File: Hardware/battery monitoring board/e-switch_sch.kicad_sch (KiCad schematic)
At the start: 8 parts, among them J5 Conn_01x02, K1 Relay_SPST-NO, Q2 PN2222A

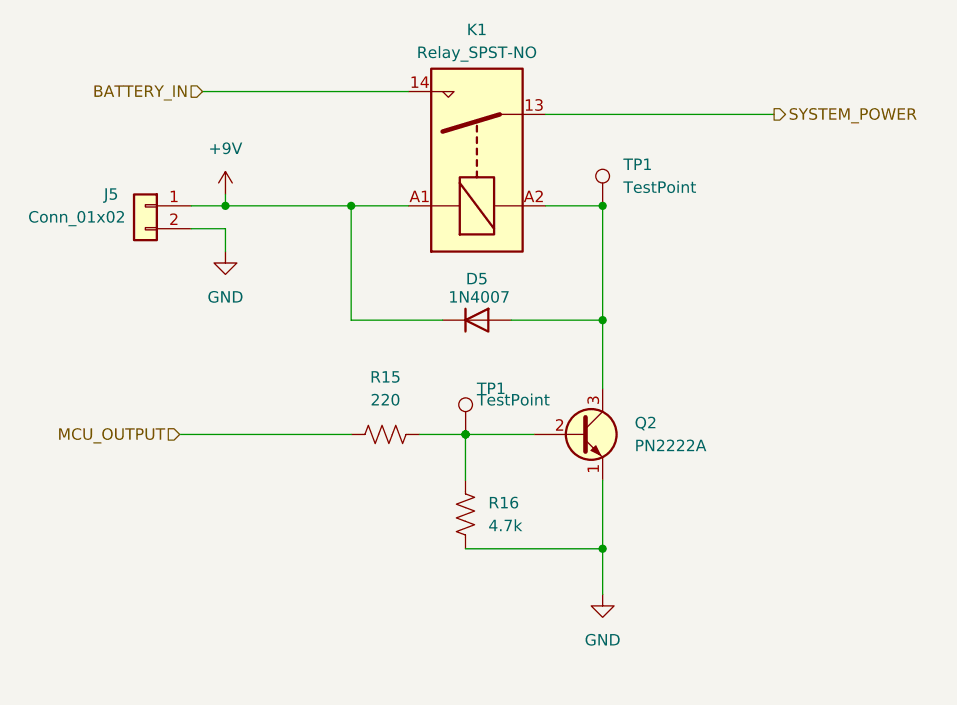
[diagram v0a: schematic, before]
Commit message: updated battery board pt.II
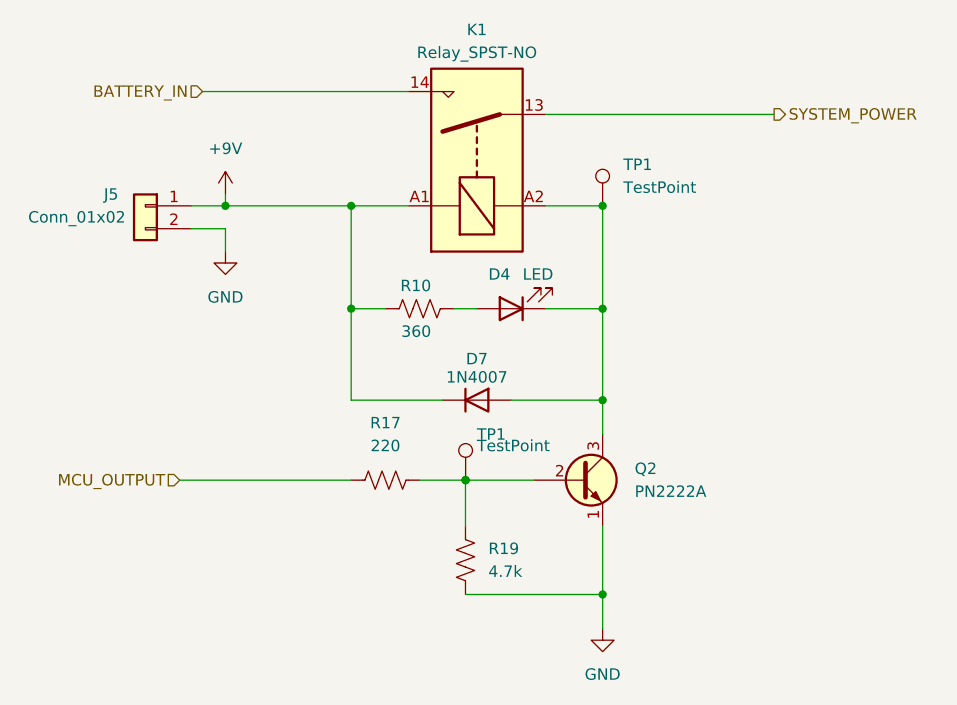
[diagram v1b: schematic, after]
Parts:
- added D4: LED, Diode_SMD:D_0805_2012Metric_Pad1.15x1.40mm_HandSolder, symbol Device:LED
- added R10: 360, Resistor_SMD:R_0805_2012Metric_Pad1.20x1.40mm_HandSolder, symbol Device:R_US
- D7: renamed from D5; footprint Diode_SMD:D_0805_2012Metric_Pad1.15x1.40mm_HandSolder -> Diode_SMD:D_SMA
- J5: footprint Library:JST_BM02B-GHS-TBT_LF__SN_ -> Library:DEANS
- TP1: footprint Library:Test Pads -> PCM_4ms_TestPoint:TestPoint_Pad_06
- renumbered R15 to R17, R16 to R19
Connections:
- net +9V: now also R10.1
- net at D7.2 (A), K1.A2, Q2.3 (C)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: now also D4.1 (K)
- new net: D4.2 (A), R10.2
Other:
- moved on the sheet: D7, Q2, R17, R19, TP1
